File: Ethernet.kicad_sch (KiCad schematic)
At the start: 7 parts, among them J2 RJ45_LINK-PP_LPJG0926HENL_Hor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, U14 TPD4EUSB30, U15 TPD4EUSB30

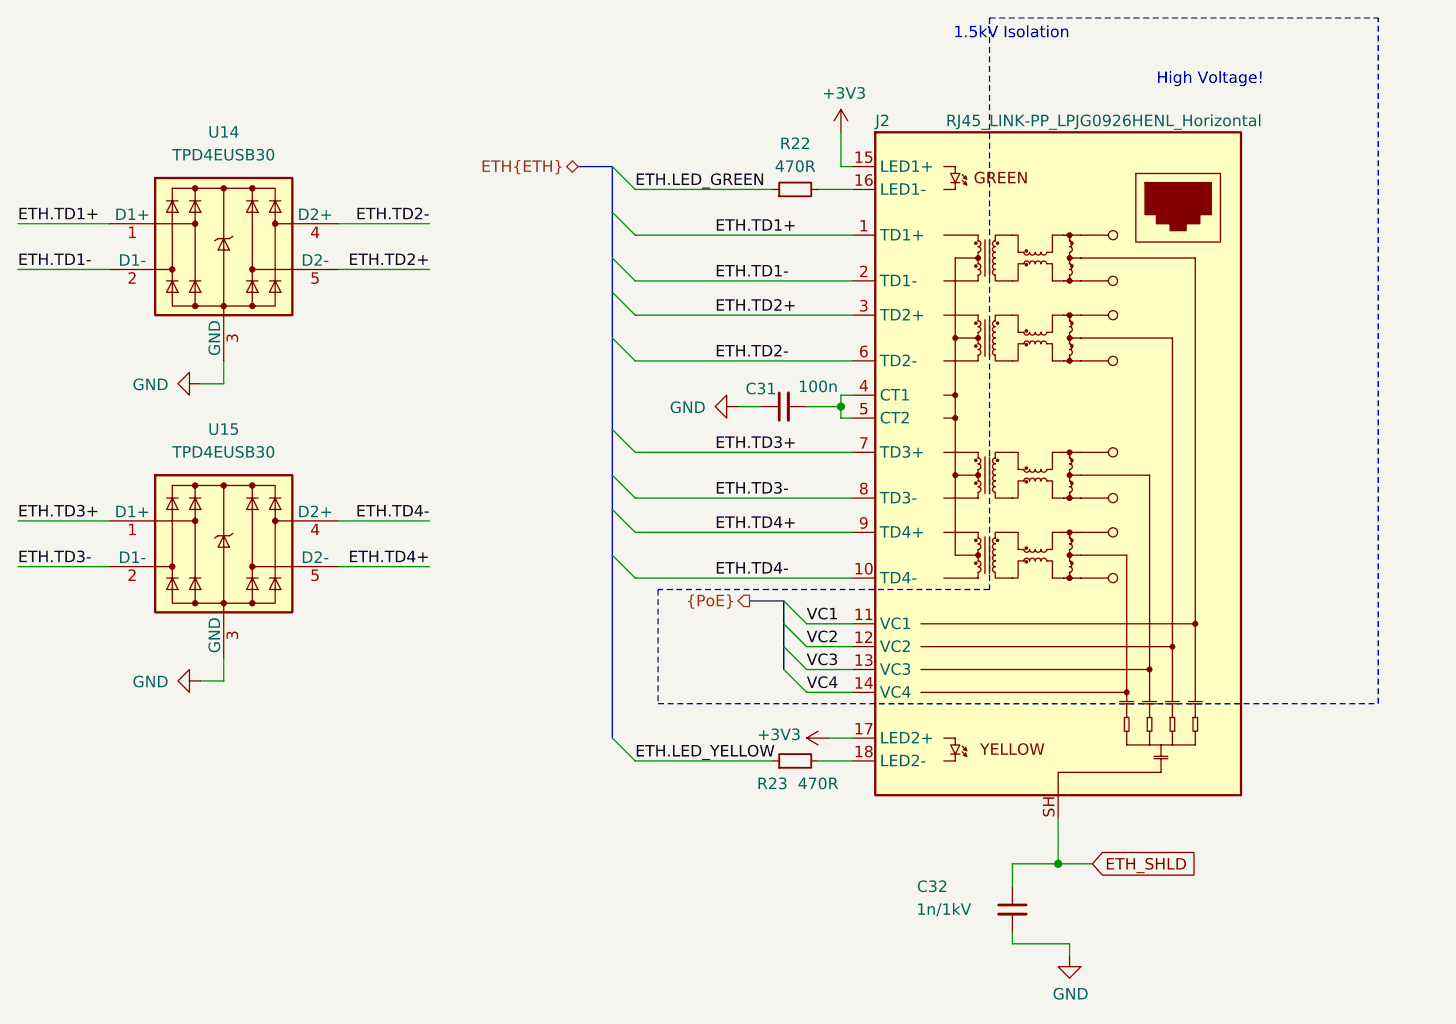
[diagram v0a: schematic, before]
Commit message: Weeded out all ERC errors
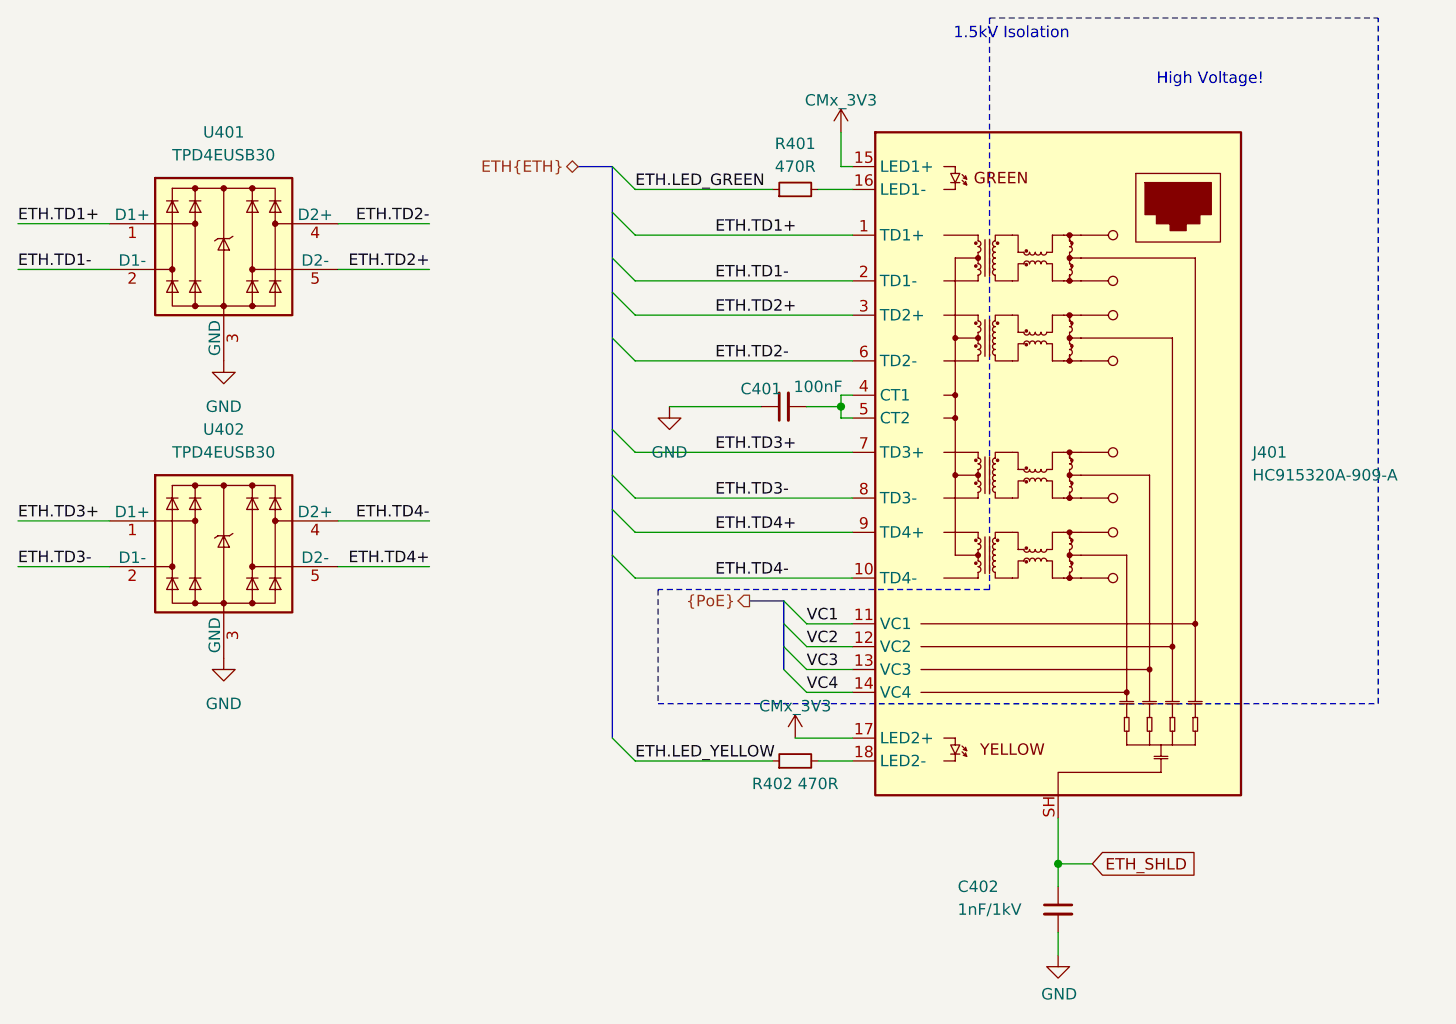
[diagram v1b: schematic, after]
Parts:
- C401: renamed from C31; value 100n -> 100nF; LCSC (none) -> C1525
- C402: renamed from C32; value 1n/1kV -> 1nF/1kV; LCSC (none) -> C1941
- J401: renamed from J2; value RJ45_LINK-PP_LPJG0926HENL_Horizontal -> HC915320A-909-A; footprint Yellow:RJ45_LINK-PP_LPJG0926HENL_Horizontal -> Hatlabs:RJ45_HC915320A-909-A_Vertical; LCSC (none) -> C5341220; Manufacturer LINK-PP -> (none); Notes (none) -> Alt. LPJG0926HENL; PartNumber LPJG0926HENL -> HC915320A-909-A
- R401: renamed from R22; LCSC (none) -> C25117
- R402: renamed from R23; LCSC (none) -> C25117
- U401: renamed from U14; LCSC (none) -> C558427
- U402: renamed from U15; LCSC (none) -> C558427; Manufacturer Texas Instruments -> (none)
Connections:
- net +3V3 renamed CMx_3V3
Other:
- company: Nabu Casa -> Hat Labs Oy
- title: Ethernet -> HALPI2
- moved on the sheet: C402
